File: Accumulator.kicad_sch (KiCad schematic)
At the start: 31 parts, among them J6 1988817, J7 1190363, J8 1190363, K1 AWHSH105D00G, K2 AWHSH105D00G, Q7 GT065P06T, Q8 IRFZ44N, U4 UCC37324P, U8 ULN2003, U9 MCP4151-xxxx-P

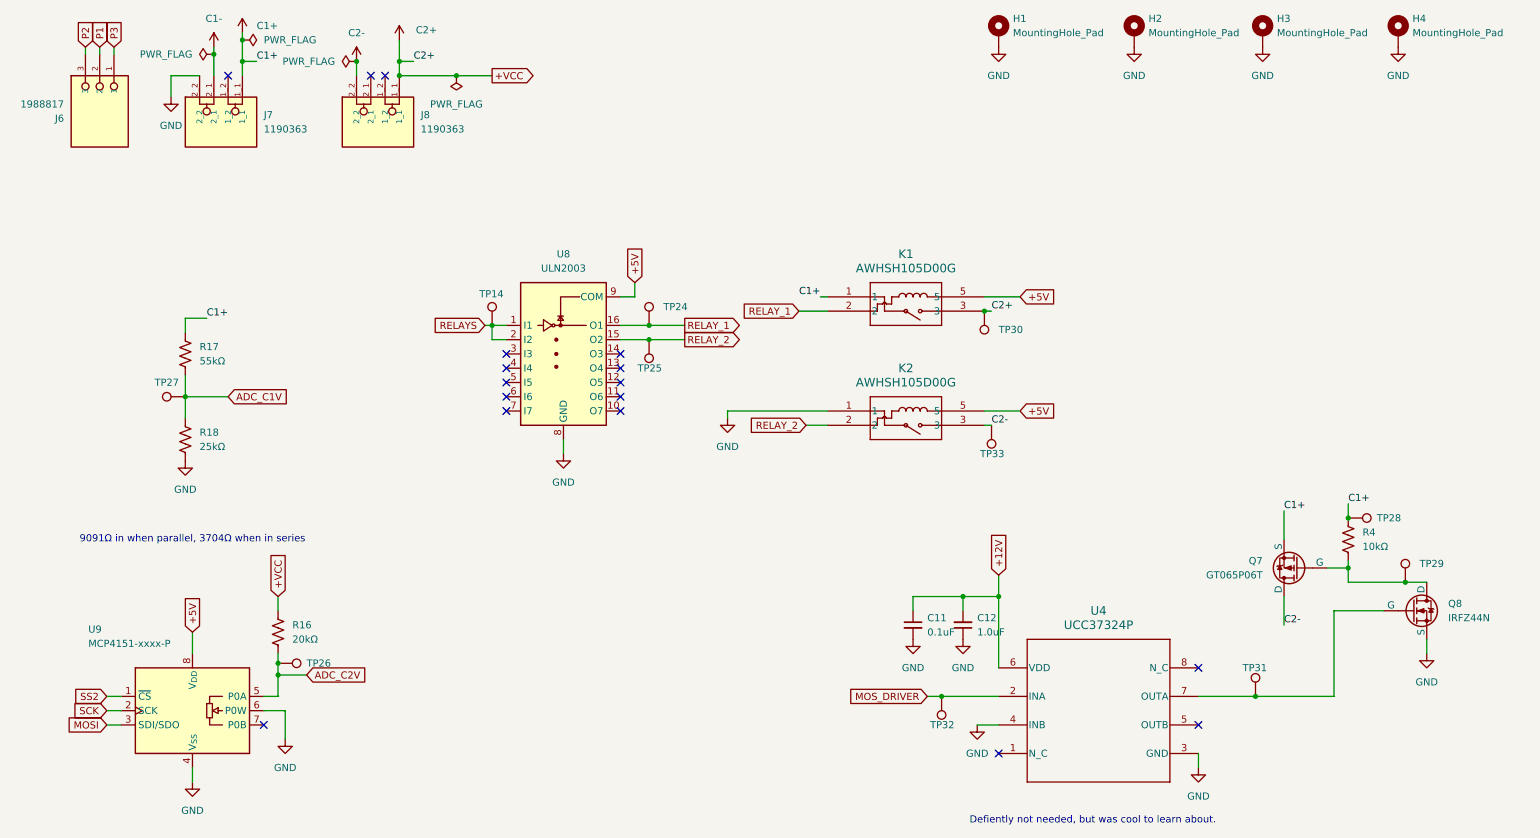
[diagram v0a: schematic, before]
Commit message: Prototyping PCB Ordered!
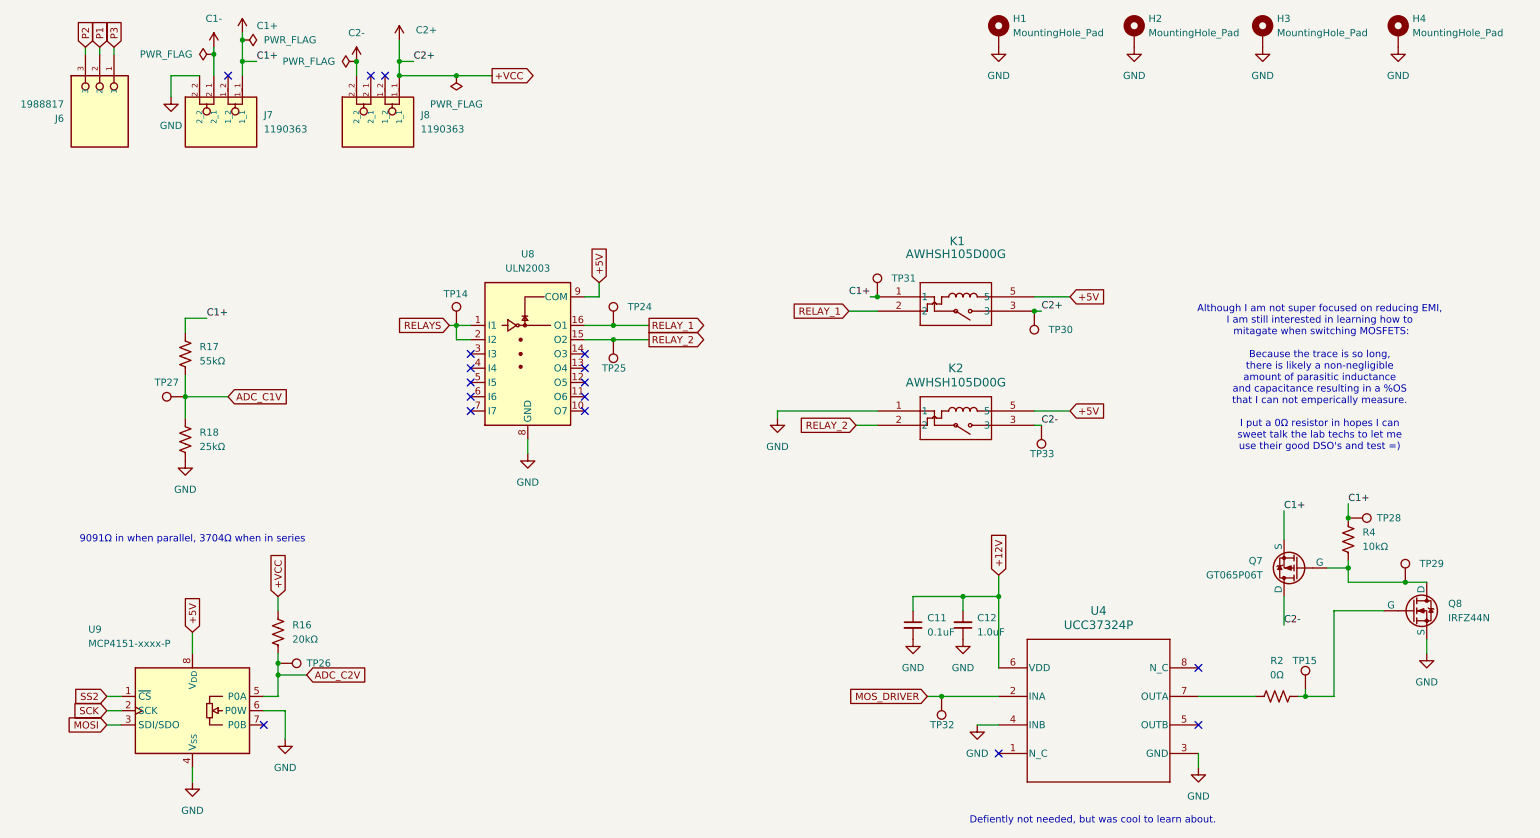
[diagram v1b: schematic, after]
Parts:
- added R2: 0Ω, Resistor_THT:R_Axial_DIN0207_L6.3mm_D2.5mm_P10.16mm_Horizontal, symbol Device:R_US
- added TP15: TestPoint, TestPoint:TestPoint_THTPad_1.0x1.0mm_Drill0.5mm, symbol Connector:TestPoint
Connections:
- net C1+: now also TP31.1
- new net: R2.1, U4.7 (OUTA)
- new net: Q8.1 (G), R2.2, TP15.1
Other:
- note added: "Although I am not super focused on reducing EMI, I am still interested in learning how to mitagate when switching MOSFETS: Because the trace is so long, there is likely a non-negligible amount of parasitic inductance and capacitance resulting in a %OS that I can not emperically measure. I put a 0Ω resistor in hopes I can sweet talk the lab techs to let me use their good DSO's and test =)"
- moved on the sheet: K1, K2, TP14, TP24, TP25, TP30, TP33, U8
